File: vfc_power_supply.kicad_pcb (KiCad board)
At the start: 4 copper layers, 160 x 160 mm, 167 parts, among them J1 Conn_01x03_Male, J2 Raspberry_Pi_4B, J3 Conn_01x02_Male, J4 Conn_01x06_Female, J5 Connector_RJ45_Magjack_Abraco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, J6 Connector_RJ45_Magjack_Abraco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, J7 Conn_01x06_Female, J8 Conn_01x06_Female, J9 Conn_01x06_Female, M1 Logo_10mmx10mm, U1 LT8653S, U10 ADS7924, U11 PCT2075D, U12 VO615A, U13 VO615A, U14 VO615A, U15 VO615A, U16 VO615A, U17 VO615A, U2 LT8636, U3 FPF2701MPX, U4 FPF2701MPX, U5 LM4040DBZ-3, U6 ISO1540, U7 ADS7924, U8 LM3480-3.3, U9 LM4040DBZ-3

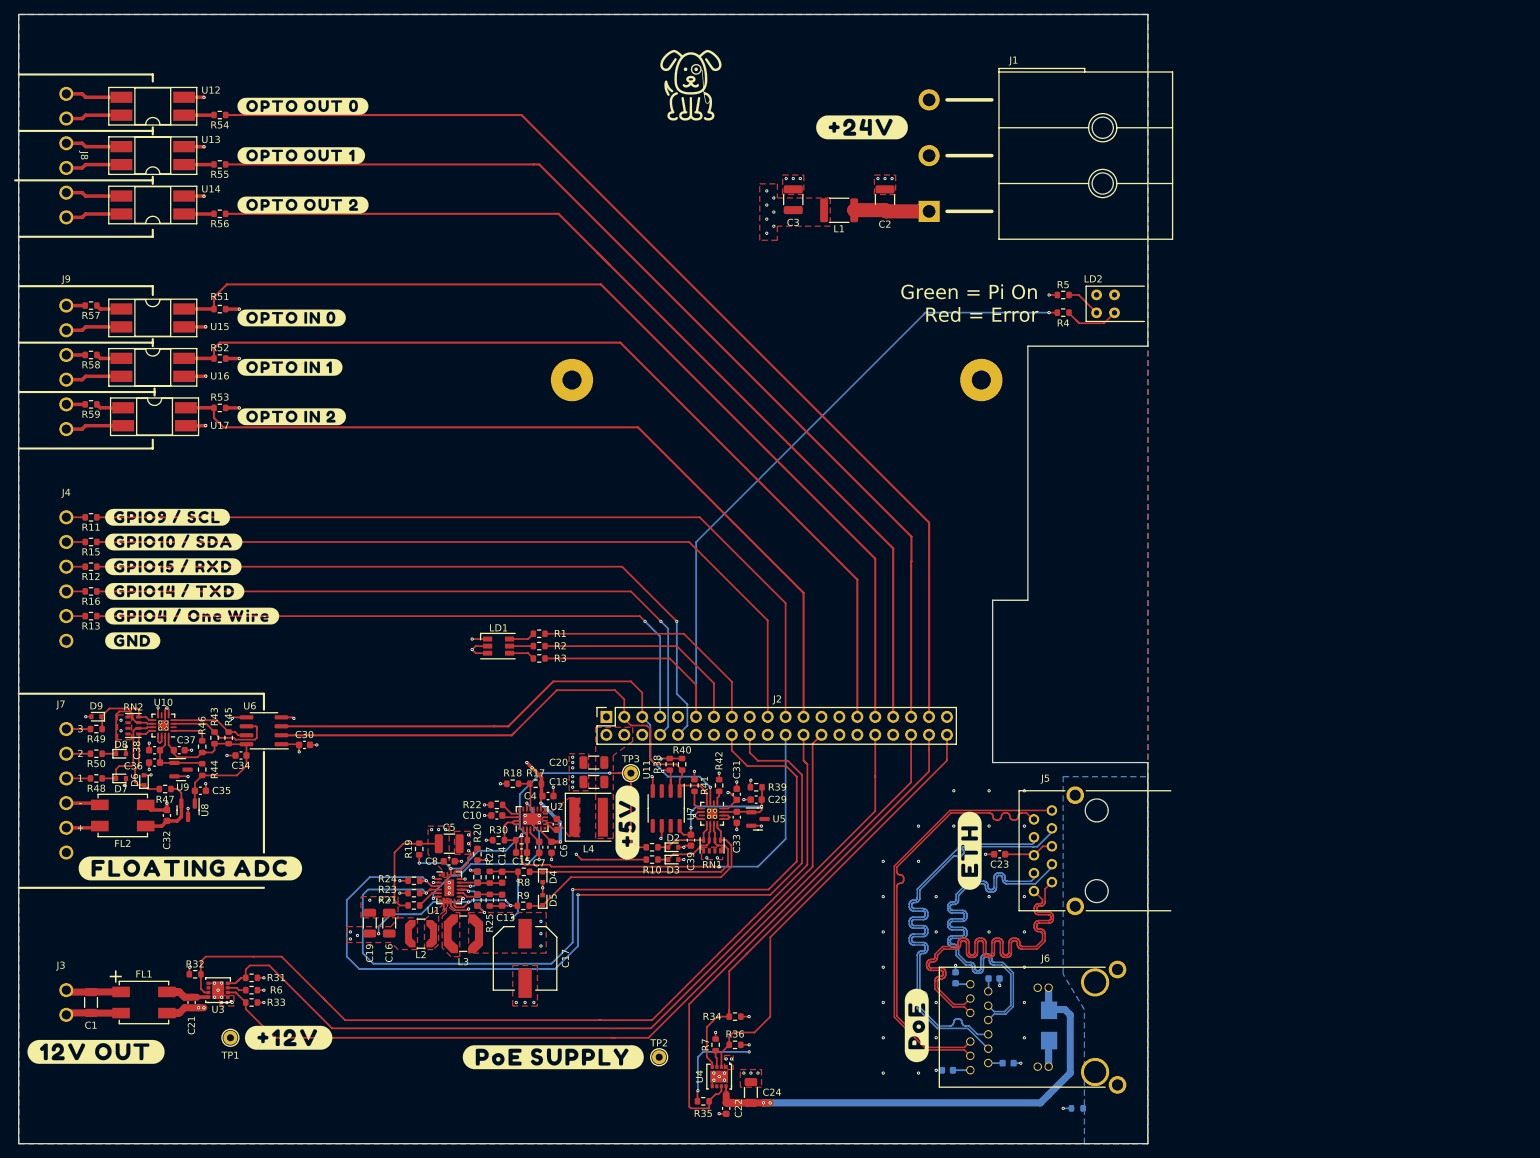
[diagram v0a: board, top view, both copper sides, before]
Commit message: Ready for review
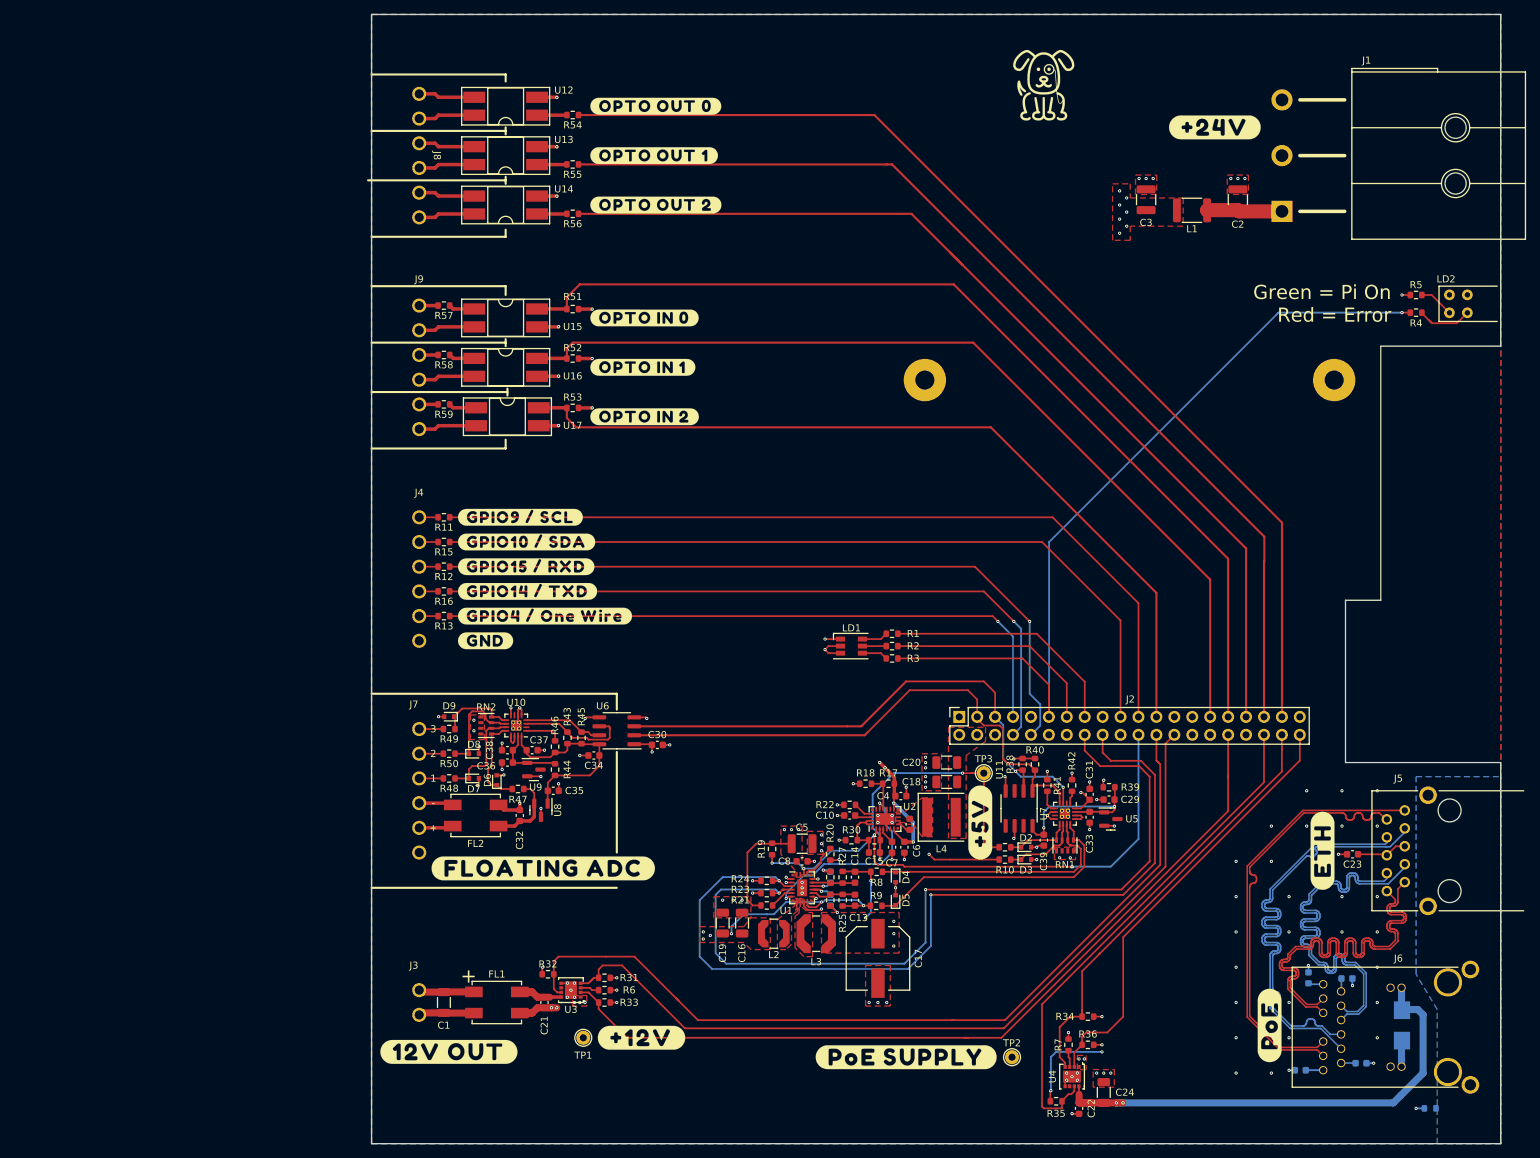
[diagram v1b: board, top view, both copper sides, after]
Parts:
- moved ? 50.0 mm to (82.2, 103.8)
- moved ? 50.0 mm to (145.8, 162.8)
- moved ? 50.0 mm to (101.0, 65.0)
- moved ? 50.0 mm to (82.2, 86.2)
- moved ? 50.0 mm to (204.8, 133.5)
- moved ? 50.0 mm to (82.2, 89.8)
- moved ? 50.0 mm to (101.0, 35.0)
- moved ? 50.0 mm to (183.0, 31.0)
- moved ? 50.0 mm to (82.2, 93.2)
- moved ? 50.0 mm to (78.5, 136.0)
- moved ? 50.0 mm to (156.2, 129.5)
- moved ? 50.0 mm to (101.0, 72.0)
- moved ? 50.0 mm to (82.2, 96.8)
- moved ? 50.0 mm to (108.2, 160.0)
- moved ? 50.0 mm to (71.2, 162.0)
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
